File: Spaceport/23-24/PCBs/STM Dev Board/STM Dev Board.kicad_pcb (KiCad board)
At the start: 2 copper layers, 58.4 x 22.9 mm, 5 parts, among them J1 693023010811, J2 614004184726, U1 STM32F103C8Tx, U2 IS66WVS4M8BLL-104NLI, U3 W25X40CLSNIG

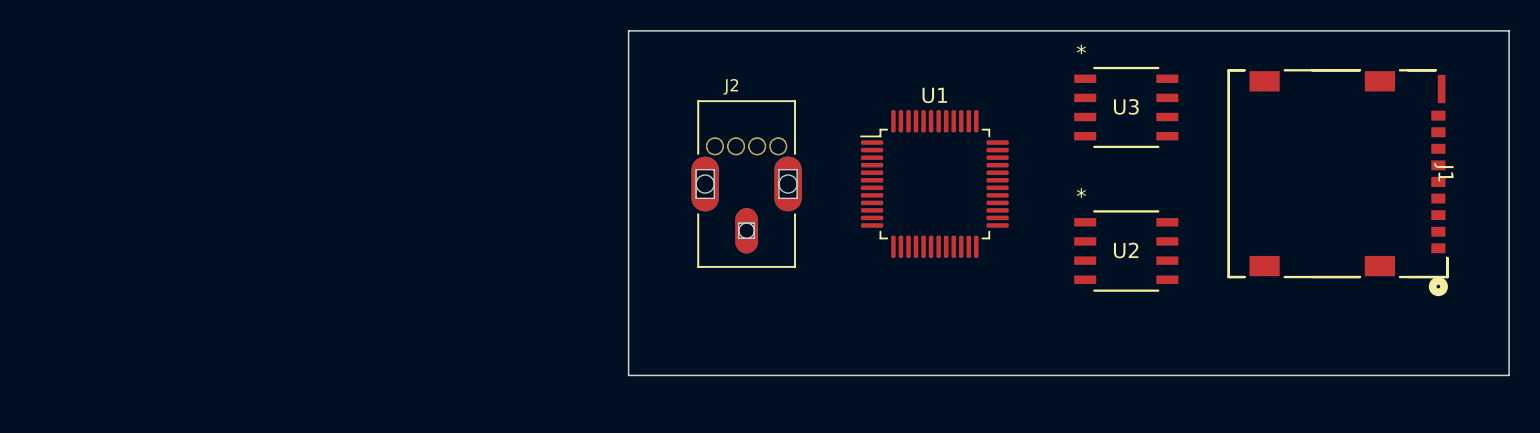
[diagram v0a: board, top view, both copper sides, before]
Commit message: Create STM Dev Board.kicad_pro
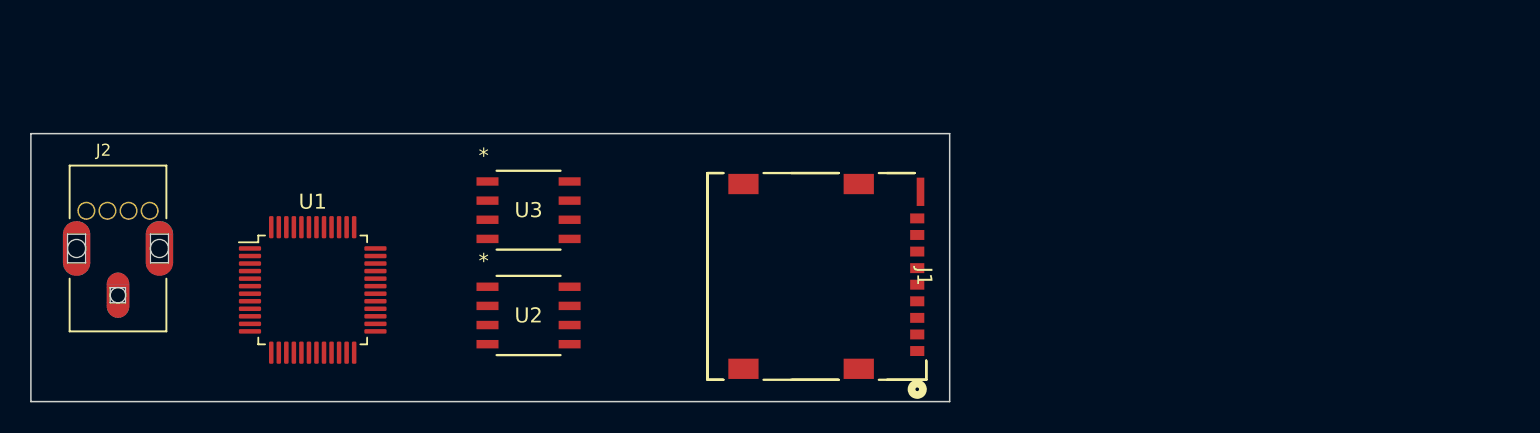
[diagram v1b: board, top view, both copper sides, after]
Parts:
- moved J2 41.9 mm to (121.1, 93.2)
- moved U1 41.9 mm to (134.0, 95.9)
- moved U3 40.2 mm to (148.3, 90.6)
- moved U2 39.9 mm to (148.3, 97.6)
- moved J1 35.2 mm to (174.1, 100.0)
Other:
- board size 58.4 x 22.9 mm -> 61 x 17.8 mm
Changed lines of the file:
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@@
   (net 78 "unconnected-(J2-SH__2-Pad7)")
   (footprint "Package_QFP:LQFP-48_7x7mm_P0.5mm" (layer "F.Cu")
-    (at 175.26 88.9)
+    (at 133.98025 95.926333)
     (descr "LQFP, 48 Pin (https://www.analog.com/media/en/technical-documentation/data-sheets/ltc2358-16.pdf), generated with kicad-footprint-generator ipc_gullwing_generator.py")
     (tags "LQFP QFP")
@@
   )
   (footprint "W25X40CLSNIG:WIN_SN-8_WIN" (layer "F.Cu")
-    (at 187.96 83.82)
+    (at 148.30275 90.636333)
     (tags "W25X40CLSNIG ")
     (property "Sheetfile" "STM Dev Board.kicad_sch")
@@
   )
   (footprint "693023010811:CONN9_3010811_WRE" (layer "F.Cu")
-    (at 208.66735 93.163669 -90)
+    (at 174.0901 99.980002 -90)
     (tags "693023010811 ")
     (property "Sheetfile" "STM Dev Board.kicad_sch")
@@
         (effects (font (size 1 1) (thickness 0.15)))
     )
-    (fp_text value "693023010811" (at 5.896331 5.46735 unlocked) (layer "F.Fab")
+    (fp_text value "693023010811" (at -6.803669 -2.15265 90 unlocked) (layer "F.Fab")
         (effects (font (size 1 1) (thickness 0.15)))
     )
@@
   )
   (footprint "USB:CONN_614004184726" (layer "F.Cu")
-    (at 162.77 88.9)
+    (at 121.06275 93.176333)
     (property "MANUFACTURER" "Wurth Electronics Inc.")
     (property "Sheetfile" "STM Dev Board.kicad_sch")
@@
         (effects (font (size 0.801465 0.801465) (thickness 0.15)))
     )
-    (fp_text value "614004184726" (at -1.84 7.66) (layer "F.Fab")
+    (fp_text value "614004184726" (at -0.21 7.66) (layer "F.Fab")
         (effects (font (size 0.800433 0.800433) (thickness 0.15)))
     )
@@
   )
   (footprint "IS66WVS4M8BLL_104NLI:SOIC8_150MIL_N_ISI" (layer "F.Cu")
-    (at 187.96 93.345)
+    (at 148.30275 97.621333)
     (tags "IS66WVS4M8BLL-104NLI ")
     (property "Sheetfile" "STM Dev Board.kicad_sch")
@@
       (net 54 "unconnected-(U2-VDD-Pad8)") (pinfunction "VDD") (pintype "power_in"))
   )
-  (gr_rect (start 154.94 78.74) (end 213.36 101.6)
+  (gr_rect (start 115.28275 85.556333) (end 176.24275 103.336333)
     (stroke (width 0.1) (type default)) (fill none) (layer "Edge.Cuts"))
 )
